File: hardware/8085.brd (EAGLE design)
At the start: 167.9 x 122.5 mm, 53 parts, among them IC10 74HCT00N, IC11 74HCT245DW, IC2 74AC573N, IC3 ATF16V8BP3, IC4 74AC00D, IC5 74HCT245DW, IC6 74AC273N, IC7 74HCT139N, IC8 7404N, IC9 74HCT138N

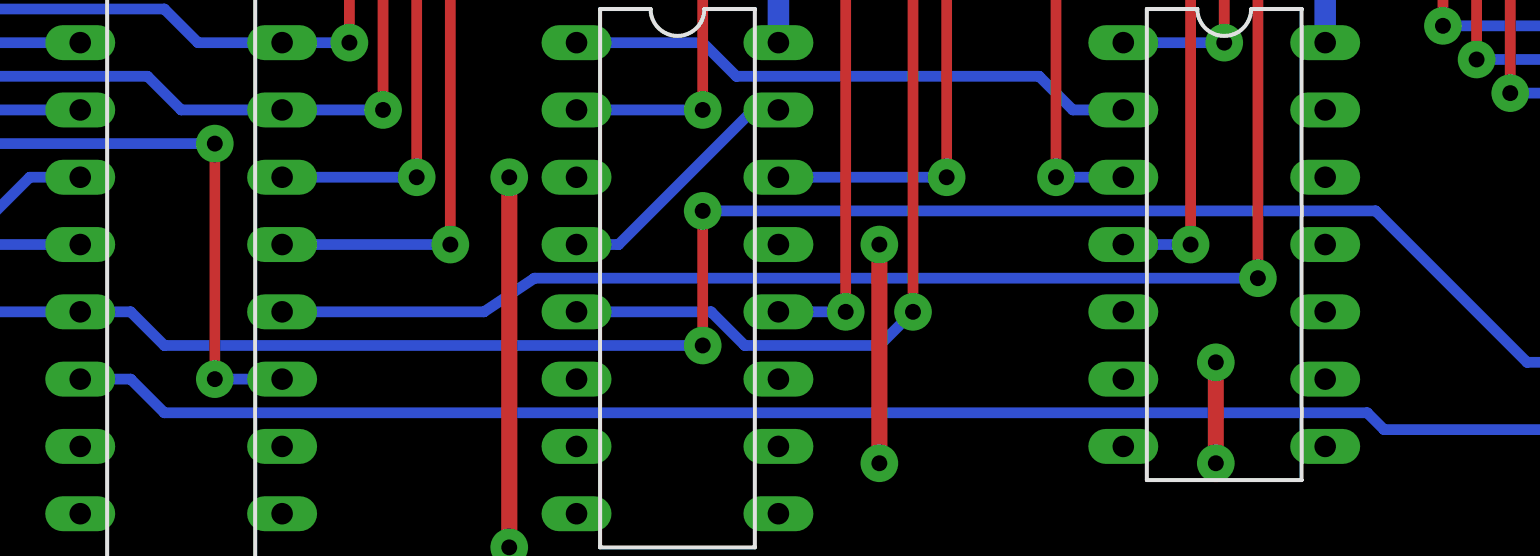
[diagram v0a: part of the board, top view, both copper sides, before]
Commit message: minor PCB change
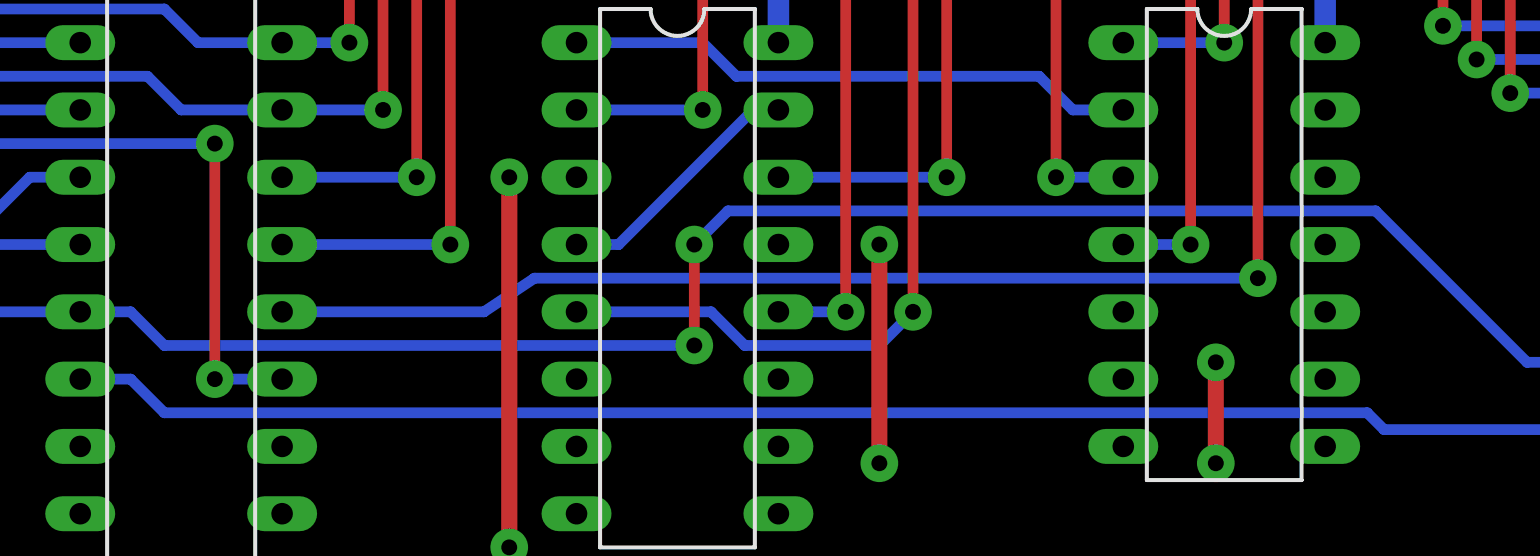
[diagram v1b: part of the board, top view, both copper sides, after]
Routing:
- net IO_M: track 173.8 -> 173.0 mm
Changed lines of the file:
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@@
 <wire x1="77.47" y1="14.605" x2="79.375" y2="14.605" width="0.4064" layer="16"/>
 <wire x1="79.375" y1="14.605" x2="80.645" y2="13.335" width="0.4064" layer="16"/>
-<wire x1="80.645" y1="13.335" x2="100.965" y2="13.335" width="0.4064" layer="16"/>
-<via x="100.965" y="13.335" extent="1-16" drill="0.6" diameter="1.4224" shape="octagon"/>
-<wire x1="100.965" y1="13.335" x2="100.965" y2="18.415" width="0.4064" layer="1"/>
-<via x="100.965" y="18.415" extent="1-16" drill="0.6" diameter="1.4224" shape="octagon"/>
-<wire x1="100.965" y1="18.415" x2="126.365" y2="18.415" width="0.4064" layer="16"/>
+<wire x1="80.645" y1="13.335" x2="100.6475" y2="13.335" width="0.4064" layer="16"/>
+<via x="100.6475" y="13.335" extent="1-16" drill="0.6" diameter="1.4224" shape="octagon"/>
+<via x="100.6475" y="17.145" extent="1-16" drill="0.6" diameter="1.4224" shape="octagon"/>
 <wire x1="126.365" y1="18.415" x2="132.08" y2="12.7" width="0.4064" layer="16"/>
 <wire x1="132.08" y1="12.7" x2="140.6525" y2="12.7" width="0.4064" layer="16"/>
+<wire x1="126.365" y1="18.415" x2="101.9175" y2="18.415" width="0.4064" layer="16"/>
+<wire x1="101.9175" y1="18.415" x2="100.6475" y2="17.145" width="0.4064" layer="16"/>
+<wire x1="100.6475" y1="13.335" x2="100.6475" y2="17.145" width="0.4064" layer="1"/>
 </signal>
 <signal name="LOCAL_PORT_CS">
